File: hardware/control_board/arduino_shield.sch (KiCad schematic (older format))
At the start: 7 parts, among them P1 Digital, P2 Power, P3 Analog, P4 Analog, P5 PWM, P6 PWM, P7 Communication

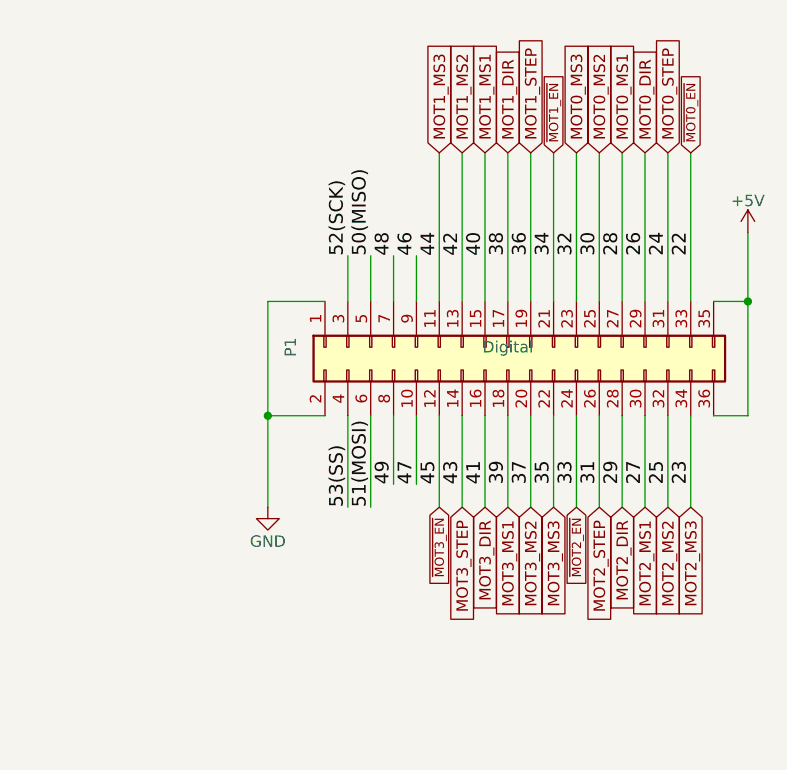
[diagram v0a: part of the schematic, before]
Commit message: add misc connectors
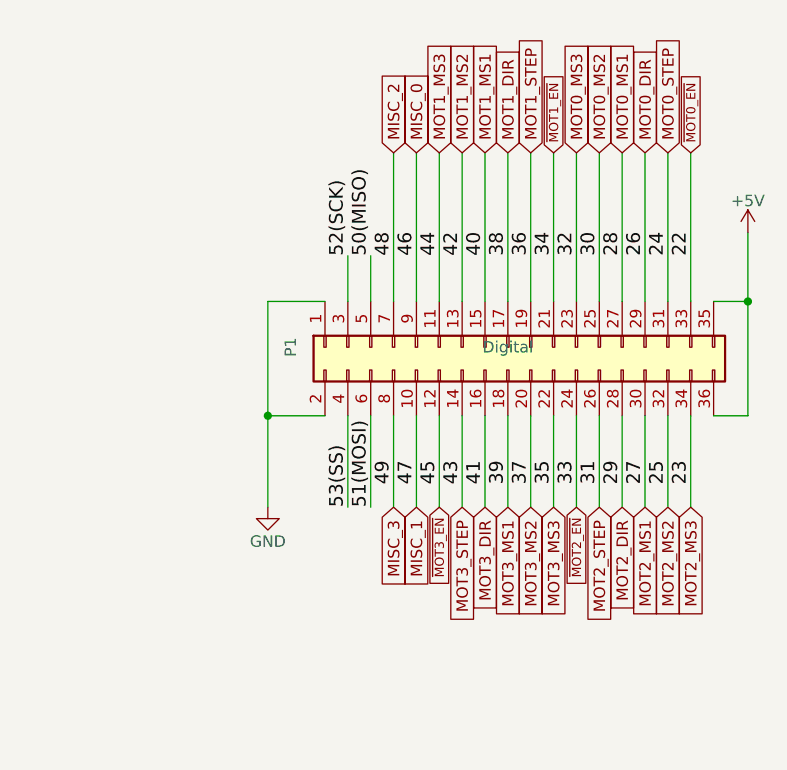
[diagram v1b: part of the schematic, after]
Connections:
- net 46 renamed MISC_0
- net 47 renamed MISC_1
- net 48 renamed MISC_2
- net 49 renamed MISC_3
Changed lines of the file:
@@
 	3800 5350 4050 5350
 Wire Wire Line
-	7800 2900 7800 2700
-Wire Wire Line
-	7700 2900 7700 2700
-Wire Wire Line
 	7600 2900 7600 2700
 Wire Wire Line
 	7500 2900 7500 2700
-Wire Wire Line
-	7800 3400 7800 3700
-Wire Wire Line
-	7700 3400 7700 3700
 Wire Wire Line
 	7600 3400 7600 3800
@@
 Wire Wire Line
 	3800 2900 4400 2900
+Text GLabel 7800 2250 1    50   Input ~ 0
+MISC_0
+Text GLabel 7700 2250 1    50   Input ~ 0
+MISC_2
+Text GLabel 7800 3800 3    50   Input ~ 0
+MISC_1
+Text GLabel 7700 3800 3    50   Input ~ 0
+MISC_3
+Wire Wire Line
+	7700 3400 7700 3800
+Wire Wire Line
+	7800 3400 7800 3800
+Wire Wire Line
+	7800 2250 7800 2900
+Wire Wire Line
+	7700 2250 7700 2900
 $EndSCHEMATC
